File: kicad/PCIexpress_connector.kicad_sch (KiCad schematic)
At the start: 10 parts, among them J1 PCIexpress_bracket, J2 PCIexpress_x4, U1 TPD4E02B04DQA, U2 TPD4E02B04DQA, U3 TPD4E02B04DQA, U4 TPD4E02B04DQA, U5 TPD4E02B04DQA, U6 TPD4E02B04DQA, U7 TPD4E02B04DQA, U8 TPD4E02B04DQA

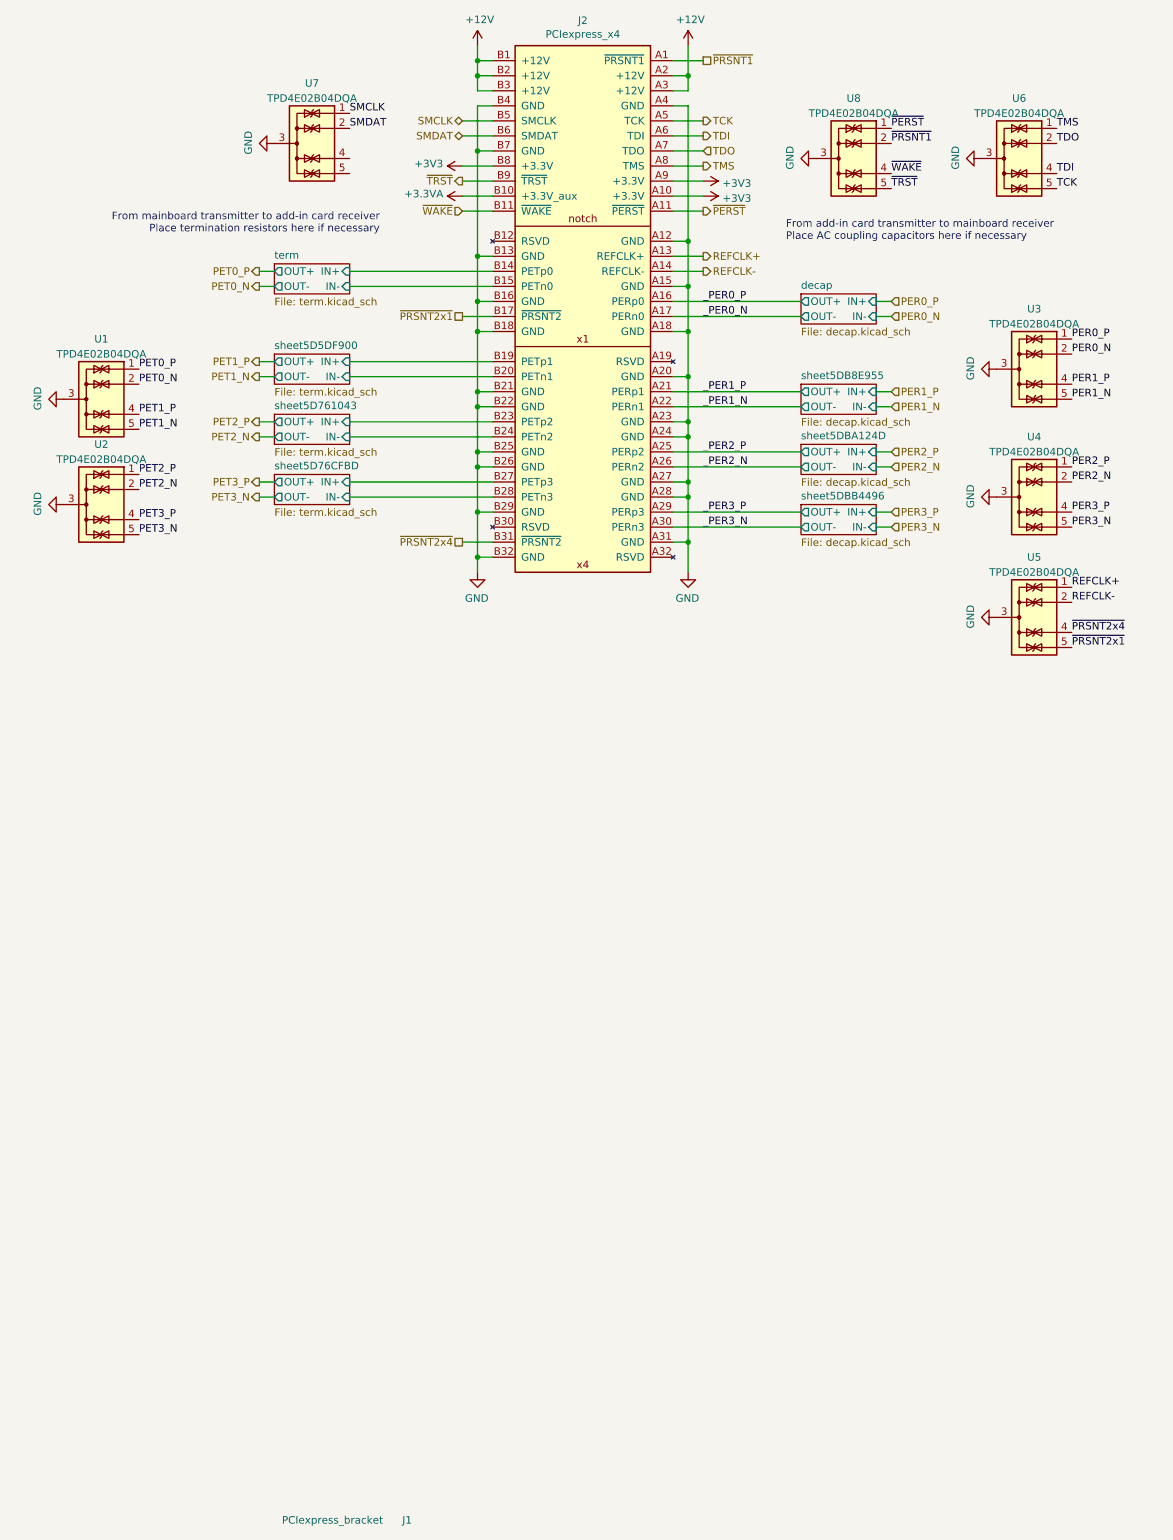
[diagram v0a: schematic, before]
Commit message: uređena schema
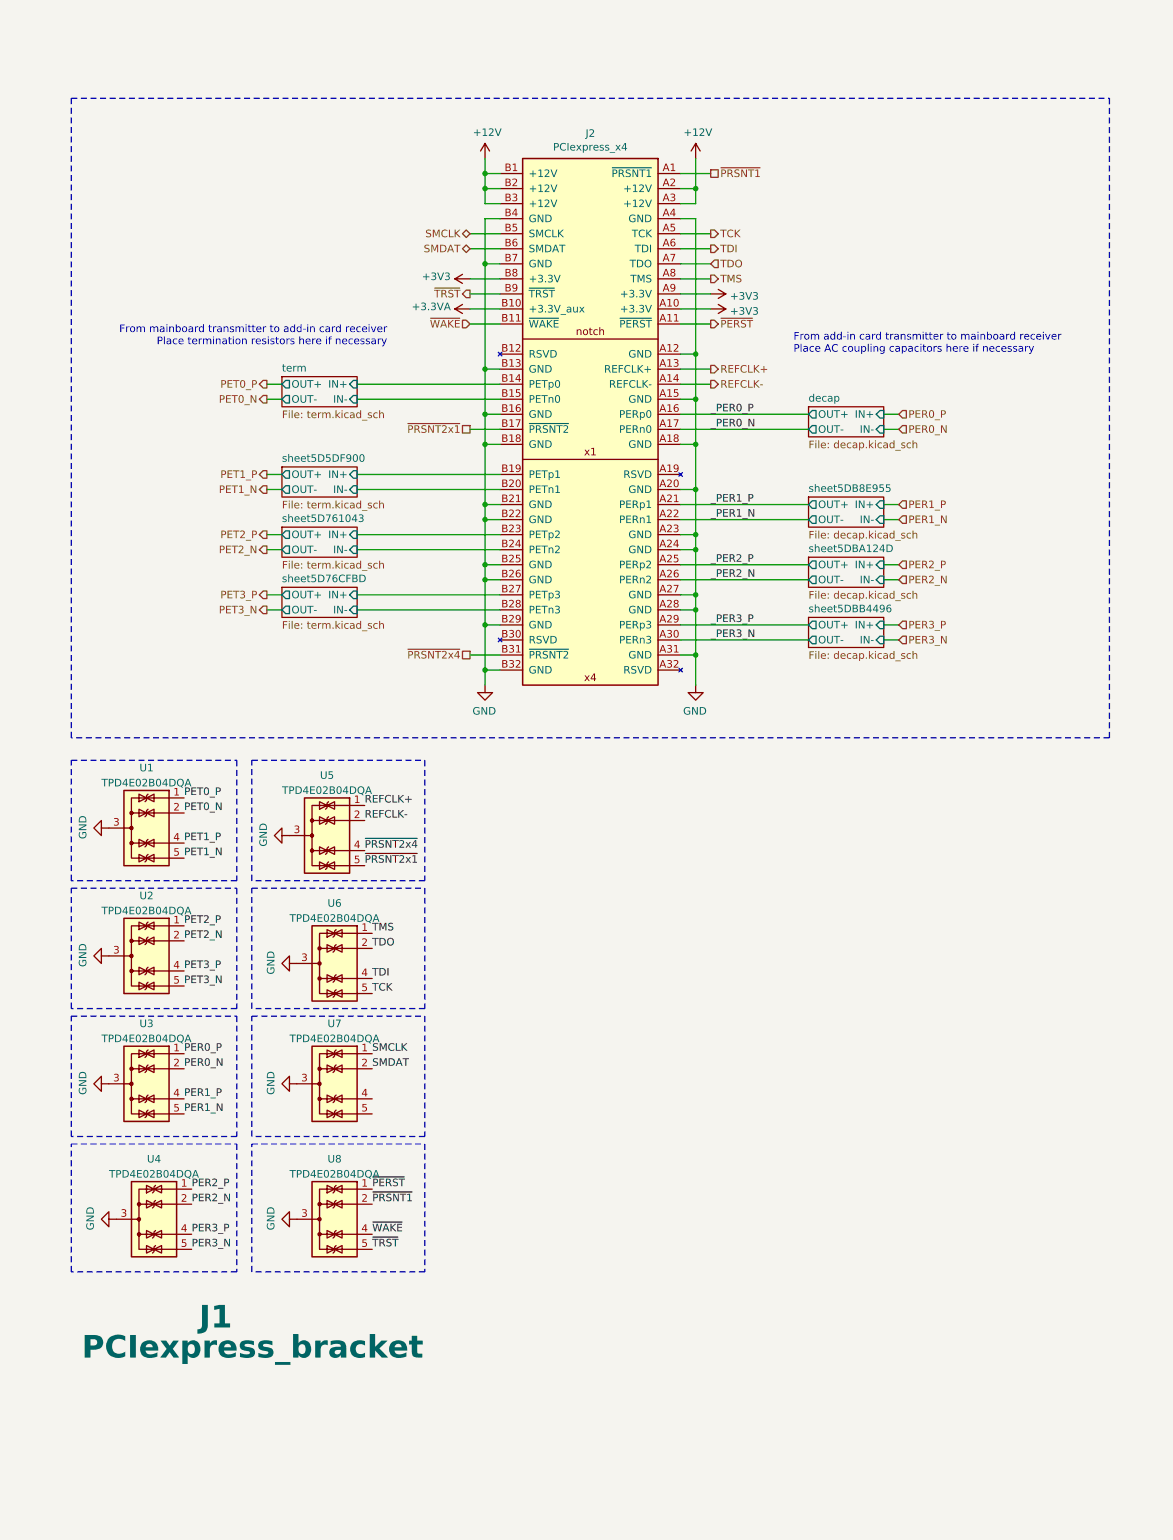
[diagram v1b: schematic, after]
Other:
- company: Author: Luca Anastasio -> ${project_creator}
- title: PCIexpress_x4_half -> ${project_name} ${project_version}
- moved on the sheet: J2, U1, U2, U3, U4, U5, U6, U7, U8
